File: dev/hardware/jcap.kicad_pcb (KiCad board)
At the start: 2 copper layers, 188 x 79.5 mm, 74 parts, among them J201 CPU PGMR, J202 GPU PGMR, J203 SPARE GPU HDR, J204 SPARE CPU HDR, J301 DC IN, J502 VGA OUT, J601 CONTROLS, SW201 CPU ~{RES}, SW202 GPU ~{RES}, SW203 DEBUG, SW601 TILT, U101 P8X32A-D40, U201 P8X32A-D40, U302 LF33_TO220, U401 24LC256, U402 24LC256, U601 74HC165, U602 74HC165, Y101 6.5MHz, Y201 6.5MHz

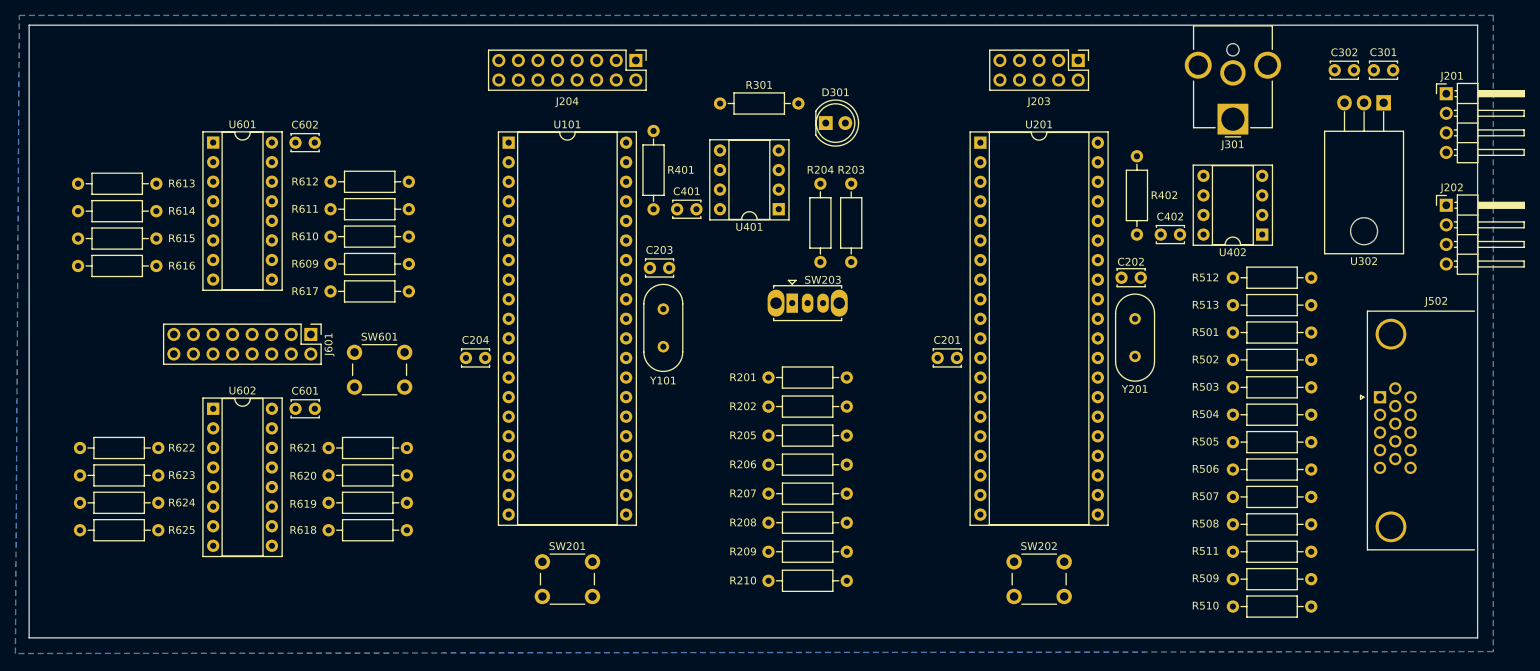
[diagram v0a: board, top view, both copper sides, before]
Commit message: Finished draft PCB
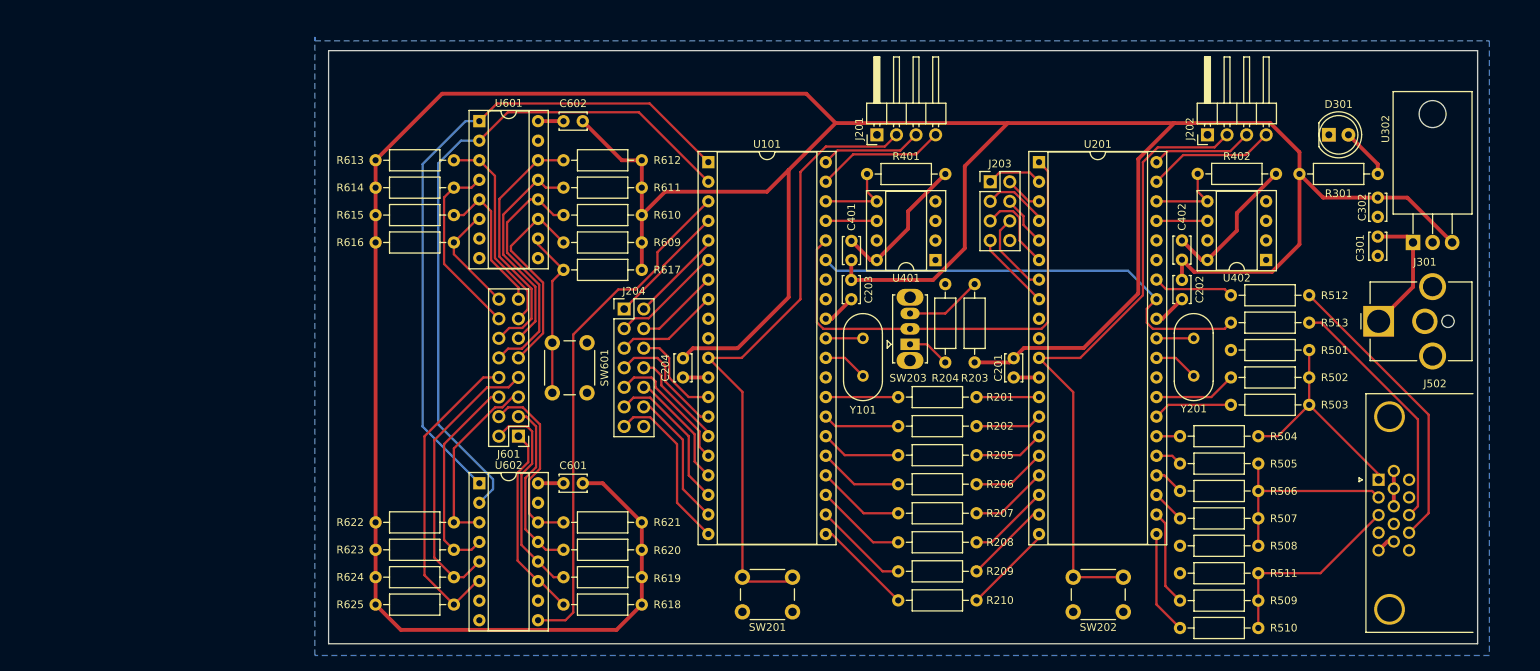
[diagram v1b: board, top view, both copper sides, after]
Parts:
- J203: footprint Connector_PinHeader_2.54mm:PinHeader_2x05_P2.54mm_Vertical -> Connector_PinHeader_2.54mm:PinHeader_2x04_P2.54mm_Vertical
- J204: footprint Connector_PinHeader_2.54mm:PinHeader_2x08_P2.54mm_Vertical -> Connector_PinHeader_2.54mm:PinHeader_2x07_P2.54mm_Vertical
- moved R301 75.7 mm to (215.6, 81.5)
- moved J201 74.1 mm to (160.8, 76.5), turned to 90 degrees
- moved D301 65.3 mm to (219.5, 76.5)
- moved R622 39.5 mm to (105.9, 126.7)
- moved R623 39.5 mm to (105.9, 130.3)
- moved R624 39.5 mm to (105.9, 133.9)
- moved R625 39.5 mm to (105.9, 137.4)
- moved R613 38.7 mm to (105.9, 79.8)
- moved R614 38.7 mm to (105.9, 83.3)
- moved R615 38.7 mm to (105.9, 86.9)
- moved R616 38.7 mm to (105.9, 90.4)
- moved C601 36.1 mm to (120.1, 121.7)
- moved U602 35.9 mm to (109.2, 121.7)
- moved C602 34.9 mm to (120.1, 74.7)
- moved U601 34.6 mm to (109.2, 74.7)
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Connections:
- J203 pad 8: /Propellers/GPU_SPARE_8 -> unconnected-(J203-Pin_8-Pad8)
- J204 pad 14: /Propellers/CPU_SPARE_14 -> unconnected-(J204-Pin_14-Pad14)
- U101 pad 13: /Propellers/CPU_SPARE_8 -> /Propellers/CPU_SPARE_6
- U101 pad 14: /Propellers/CPU_SPARE_9 -> /Propellers/CPU_SPARE_7
- U101 pad 15: /Propellers/CPU_SPARE_10 -> /Propellers/CPU_SPARE_8
- U101 pad 16: /Propellers/CPU_SPARE_11 -> /Propellers/CPU_SPARE_9
- U101 pad 17: /Propellers/CPU_SPARE_12 -> /Propellers/CPU_SPARE_10
- U101 pad 18: /Propellers/CPU_SPARE_13 -> /Propellers/CPU_SPARE_11
- U101 pad 19: /Propellers/CPU_SPARE_14 -> /Propellers/CPU_SPARE_12
- U101 pad 20: /Propellers/CPU_SPARE_15 -> /Propellers/CPU_SPARE_13
- U101 pad 33: /Propellers/CPU_SPARE_1 -> unconnected-(U101-P24-Pad33)
- U101 pad 34: /Propellers/CPU_SPARE_2 -> unconnected-(U101-P25-Pad34)
- U101 pad 4: /Propellers/CPU_SPARE_3 -> /Propellers/CPU_SPARE_1
- U101 pad 5: /Propellers/CPU_SPARE_4 -> /Propellers/CPU_SPARE_2
- U101 pad 6: /Propellers/CPU_SPARE_5 -> /Propellers/CPU_SPARE_3
- U101 pad 7: /Propellers/CPU_SPARE_6 -> /Propellers/CPU_SPARE_4
- U101 pad 8: /Propellers/CPU_SPARE_7 -> /Propellers/CPU_SPARE_5
- U201 pad 2: /Propellers/GPU_SPARE_3 -> /Propellers/GPU_SPARE_1
- U201 pad 3: /Propellers/GPU_SPARE_4 -> /Propellers/GPU_SPARE_2
- U201 pad 35: /Propellers/GPU_SPARE_1 -> unconnected-(U201-P26-Pad35)
- U201 pad 36: /Propellers/GPU_SPARE_2 -> unconnected-(U201-P27-Pad36)
- U201 pad 4: /Propellers/GPU_SPARE_5 -> /Propellers/GPU_SPARE_3
- U201 pad 5: /Propellers/GPU_SPARE_6 -> /Propellers/GPU_SPARE_4
- U201 pad 6: /Propellers/GPU_SPARE_7 -> /Propellers/GPU_SPARE_5
- U201 pad 7: /Propellers/GPU_SPARE_8 -> /Propellers/GPU_SPARE_6
- U201 pad 8: /Propellers/GPU_SPARE_9 -> /Propellers/GPU_SPARE_7
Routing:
- net +3.3V: track 0.00 -> 471.6 mm
- net INPUTS_CLK: track 0.00 -> 89.3 mm
- net ~{INPUTS_PL}: track 0.00 -> 88.0 mm
- net /Propellers/~{SER_RES_CPU}: track 0.00 -> 83.4 mm
- net /Propellers/~{SER_RES_GPU}: track 0.00 -> 83.3 mm
- net INPUTS: track 0.00 -> 66.9 mm
- net /Propellers/DEBUG: track 0.00 -> 63.1 mm
- net V_SYNC: track 0.00 -> 60.2 mm
- net /Input/IN8: track 0.00 -> 40.8 mm
- net Net-(J502-Pad14): track 0.00 -> 38.3 mm
- net /Input/IN7: track 0.00 -> 37.3 mm
- net /Input/IN12: track 0.00 -> 33.0 mm
- net Net-(J502-Pad13): track 0.00 -> 32.2 mm
- net /Input/IN10: track 0.00 -> 31.9 mm
- net /VGA_DAC/RED_OUT: track 0.00 -> 28.8 mm
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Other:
- board size 188 x 79.5 mm -> 149.1 x 77 mm
- board text added: "U302"
